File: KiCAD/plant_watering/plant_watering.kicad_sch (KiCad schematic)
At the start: 17 parts, among them J1 Barrel_Jack, P1 USB_C_Plug_USB2.0, SW1 SW_Push, SW2 SW_Push, SW3 SW_Push, SW4 SW_Push, U1 LCD-016N002L, U2 ESP32-WROOM-32

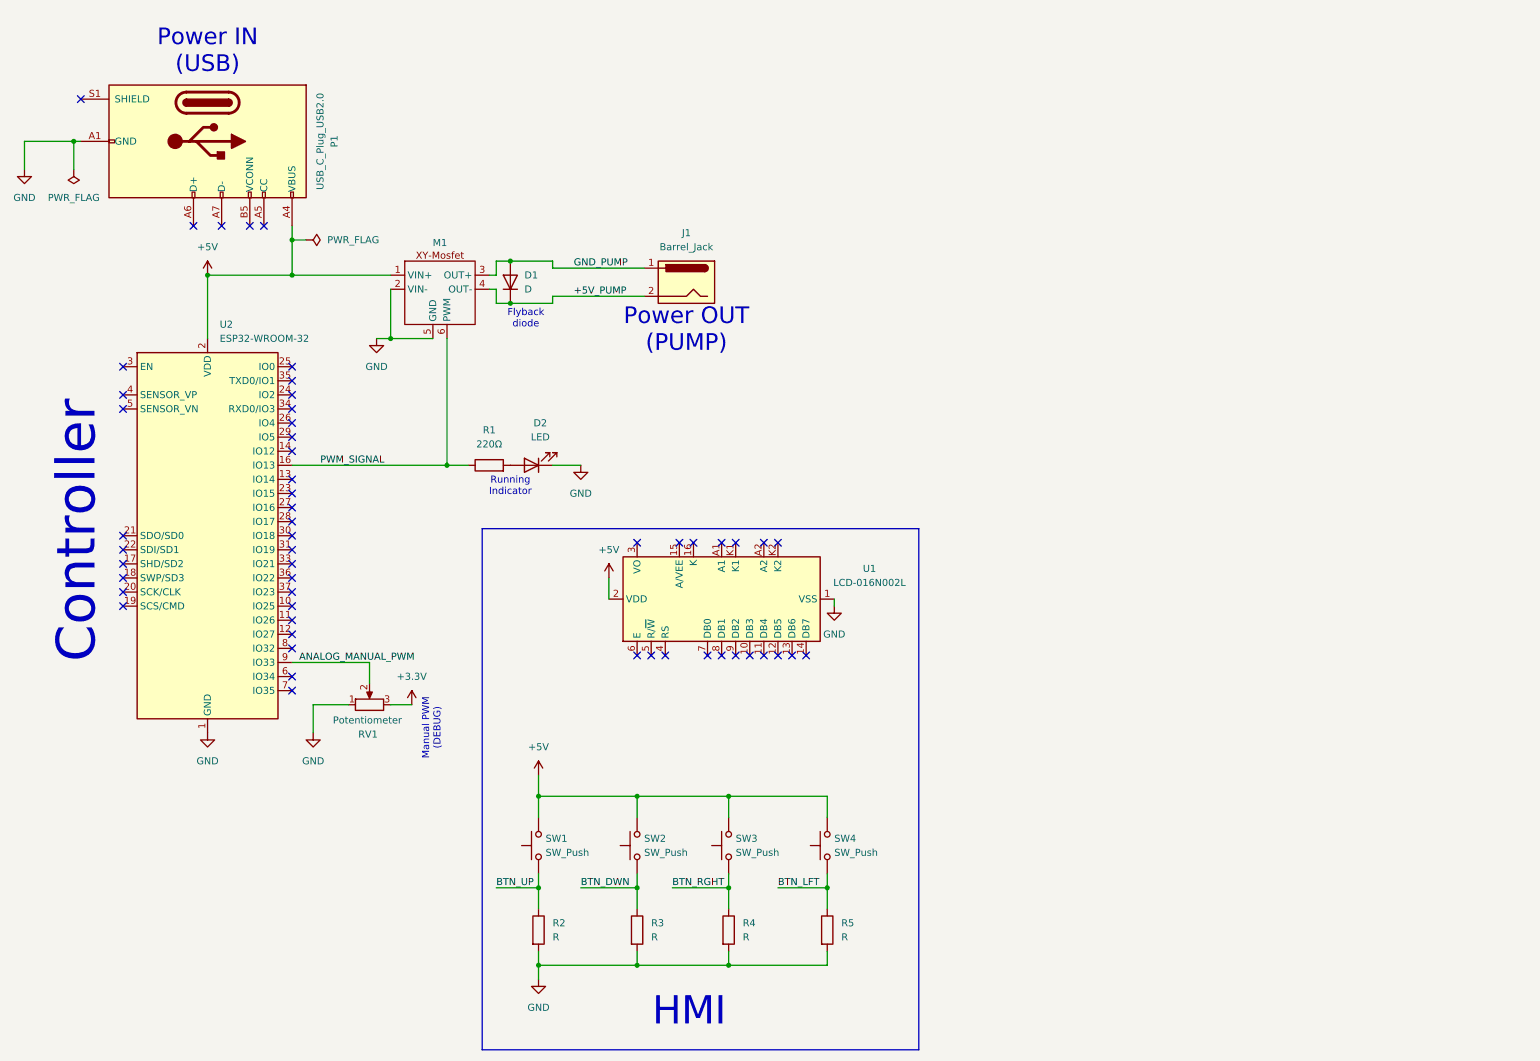
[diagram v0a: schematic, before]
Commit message: API Exchange
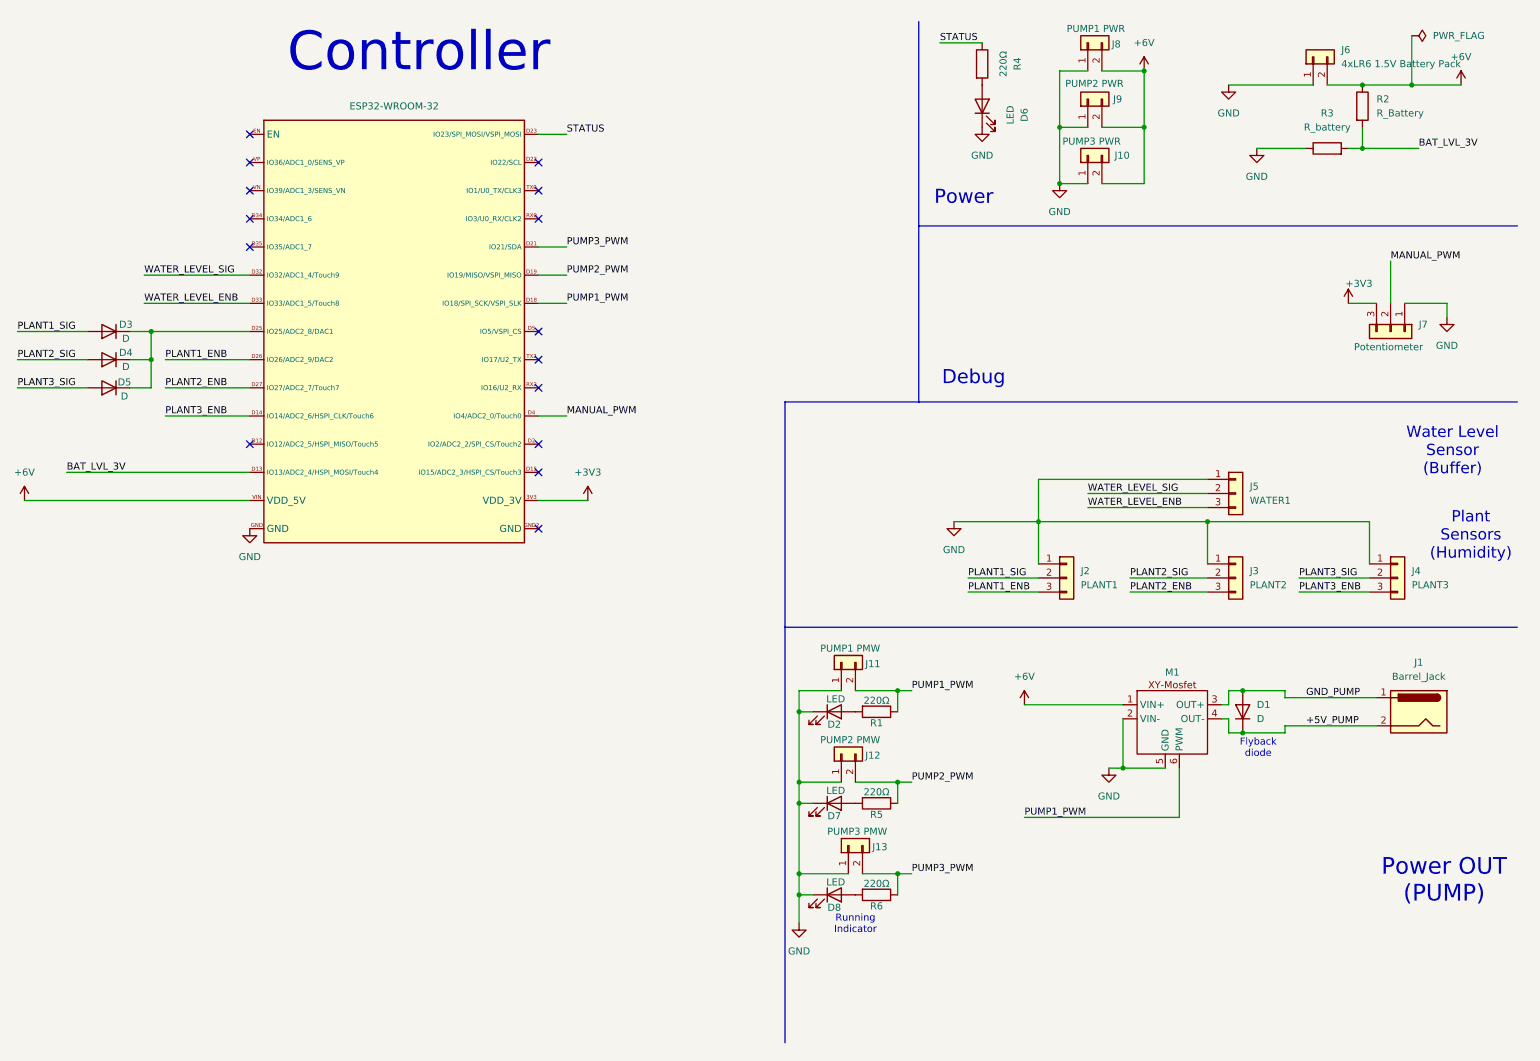
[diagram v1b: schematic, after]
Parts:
- removed P1: USB_C_Plug_USB2.0, symbol Connector:USB_C_Plug_USB2.0
- removed RV1: Potentiometer, symbol Device:R_Potentiometer
- removed SW1, SW2, SW3, SW4: SW_Push, symbol Switch:SW_Push
- removed U1: LCD-016N002L, Display:LCD-016N002L, symbol Display_Character:LCD-016N002L
- removed U2: ESP32-WROOM-32, RF_Module:ESP32-WROOM-32, symbol RF_Module:ESP32-WROOM-32
- added D3, D4, D5: D, Diode_THT:D_5W_P10.16mm_Horizontal, symbol Device:D
- added D6, D7, D8: LED, LED_THT:LED_D3.0mm, symbol Device:LED
- added J10: PUMP3 PWR, Connector_JST:JST_XH_B2B-XH-A_1x02_P2.50mm_Vertical, symbol Connector_Generic:Conn_01x02
- added J11: PUMP1 PMW, Connector_JST:JST_XH_B2B-XH-A_1x02_P2.50mm_Vertical, symbol Connector_Generic:Conn_01x02
- added J12: PUMP2 PMW, Connector_JST:JST_XH_B2B-XH-A_1x02_P2.50mm_Vertical, symbol Connector_Generic:Conn_01x02
- added J13: PUMP3 PMW, Connector_JST:JST_XH_B2B-XH-A_1x02_P2.50mm_Vertical, symbol Connector_Generic:Conn_01x02
- added J2: PLANT1, Connector_JST:JST_XH_B3B-XH-A_1x03_P2.50mm_Vertical, symbol Connector_Generic:Conn_01x03
- added J3: PLANT2, Connector_JST:JST_XH_B3B-XH-A_1x03_P2.50mm_Vertical, symbol Connector_Generic:Conn_01x03
- added J4: PLANT3, Connector_JST:JST_XH_B3B-XH-A_1x03_P2.50mm_Vertical, symbol Connector_Generic:Conn_01x03
- added J5: WATER1, Connector_JST:JST_XH_B3B-XH-A_1x03_P2.50mm_Vertical, symbol Connector_Generic:Conn_01x03
- added J6: 4xLR6 1.5V Battery Pack, Connector_JST:JST_XH_B2B-XH-A_1x02_P2.50mm_Vertical, symbol Connector_Generic:Conn_01x02
- added J7: Potentiometer, Connector_JST:JST_XH_B3B-XH-A_1x03_P2.50mm_Vertical, symbol Connector_Generic:Conn_01x03
- added J8: PUMP1 PWR, Connector_JST:JST_XH_B2B-XH-A_1x02_P2.50mm_Vertical, symbol Connector_Generic:Conn_01x02
- added J9: PUMP2 PWR, Connector_JST:JST_XH_B2B-XH-A_1x02_P2.50mm_Vertical, symbol Connector_Generic:Conn_01x02
- added R6: 220Ω, Resistor_THT:R_Axial_DIN0207_L6.3mm_D2.5mm_P10.16mm_Horizontal, symbol Device:R
- added U1: ESP32-WROOM-32, Meltwin:ESP32-C3-DevKitM-1, symbol Meltwin:ESP32-WROOM-32
- D2: footprint (none) -> LED_THT:LED_D3.0mm
- R1: footprint (none) -> Resistor_THT:R_Axial_DIN0207_L6.3mm_D2.5mm_P10.16mm_Horizontal
- R2: value R -> R_Battery; footprint (none) -> Resistor_THT:R_Axial_DIN0207_L6.3mm_D2.5mm_P10.16mm_Horizontal
- R3: value R -> R_battery; footprint (none) -> Resistor_THT:R_Axial_DIN0207_L6.3mm_D2.5mm_P10.16mm_Horizontal
- R4, R5: value R -> 220Ω; footprint (none) -> Resistor_THT:R_Axial_DIN0207_L6.3mm_D2.5mm_P10.16mm_Horizontal
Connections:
- net BTN_DWN is gone; now on net GND: R3.1
- net BTN_UP is gone; now on net +6V: R2.1
- net GND: now also D6.1 (K), D7.1 (K), D8.1 (K), J10.1 (Pin_1), J11.1 (Pin_1), J12.1 (Pin_1), J13.1 (Pin_1), J2.1 (Pin_1), J3.1 (Pin_1), J4.1 (Pin_1), J5.1 (Pin_1), J6.1 (Pin_1), J7.1 (Pin_1), J8.1 (Pin_1), J9.1 (Pin_1), U1.GND; no longer R2.2, R3.2, R4.2, R5.2
- net +5V renamed +6V
- net +6V: now also J10.2 (Pin_2), J6.2 (Pin_2), J8.2 (Pin_2), J9.2 (Pin_2), U1.VIN (VDD_5V)
- net BTN_LFT renamed PUMP2_PWM
- net PUMP2_PWM: now also J12.2 (Pin_2), U1.D19 (IO19/MISO/VSPI_MISO)
- net BTN_RGHT renamed STATUS
- net STATUS: now also U1.D23 (IO23/SPI_MOSI/VSPI_MOSI)
- net PWM_SIGNAL renamed PUMP1_PWM
- net PUMP1_PWM: now also J11.2 (Pin_2), U1.D18 (IO18/SPI_SCK/VSPI_SLK)
- new net: D3.1 (K), D4.1 (K), D5.1 (K), U1.D25 (IO25/ADC2_8/DAC1)
- new net: D8.2 (A), R6.2
- new net: D6.2 (A), R4.2
- new net: D7.2 (A), R5.2
- new net +3V3: J7.3 (Pin_3), U1.3V3 (VDD_3V)
- new net BAT_LVL_3V: R2.2, R3.2, U1.D13 (IO13/ADC2_4/HSPI_MOSI/Touch4)
- new net MANUAL_PWM: J7.2 (Pin_2), U1.D4 (IO4/ADC2_0/Touch0)
- new net PLANT1_ENB: J2.3 (Pin_3), U1.D26 (IO26/ADC2_9/DAC2)
- new net PLANT1_SIG: D3.2 (A), J2.2 (Pin_2)
- new net PLANT2_ENB: J3.3 (Pin_3), U1.D27 (IO27/ADC2_7/Touch7)
- new net PLANT2_SIG: D4.2 (A), J3.2 (Pin_2)
- new net PLANT3_ENB: J4.3 (Pin_3), U1.D14 (IO14/ADC2_6/HSPI_CLK/Touch6)
- new net PLANT3_SIG: D5.2 (A), J4.2 (Pin_2)
- new net PUMP3_PWM: J13.2 (Pin_2), R6.1, U1.D21 (IO21/SDA)
- new net WATER_LEVEL_ENB: J5.3 (Pin_3), U1.D33 (IO33/ADC1_5/Touch8)
- new net WATER_LEVEL_SIG: J5.2 (Pin_2), U1.D32 (IO32/ADC1_4/Touch9)
- no-connect marks 54 -> 15
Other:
- note added: "Debug"
- note added: "Plant Sensors (Humidity)"
- note added: "Power"
- note added: "Water Level Sensor (Buffer)"
- note removed: "HMI"
- note removed: "Manual PWM (DEBUG)"
- note removed: "Power IN (USB)"
